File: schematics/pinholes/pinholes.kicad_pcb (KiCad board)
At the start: 2 copper layers, 42 x 10 mm, 3 parts

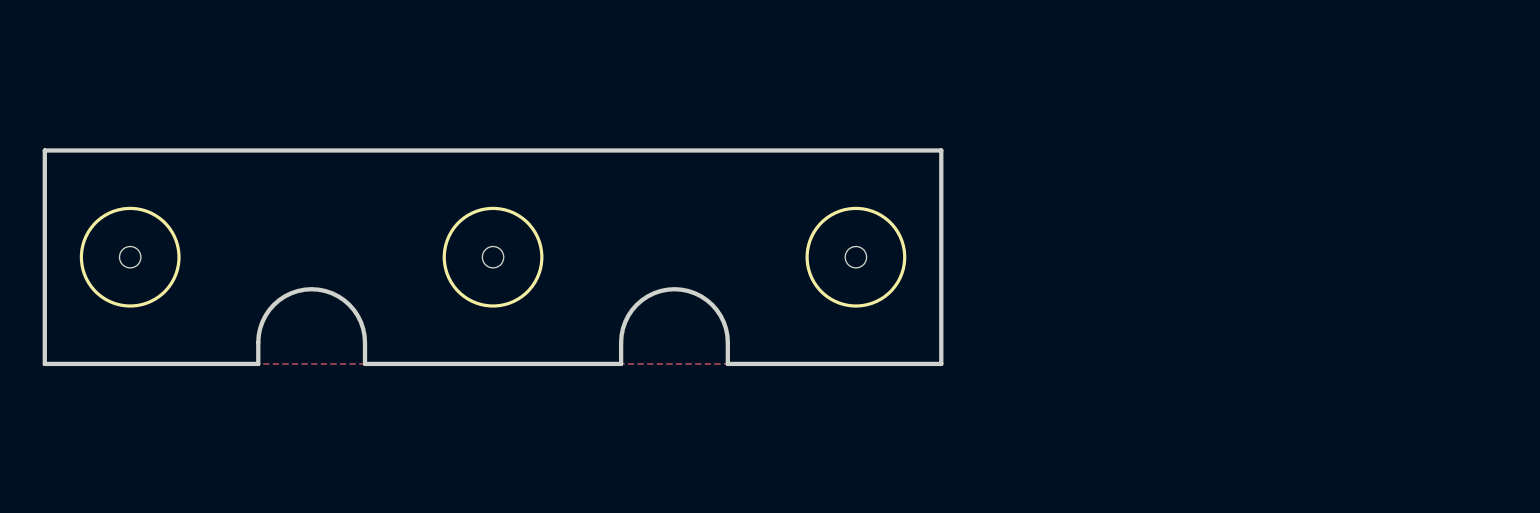
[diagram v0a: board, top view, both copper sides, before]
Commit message: Electronics update for V1
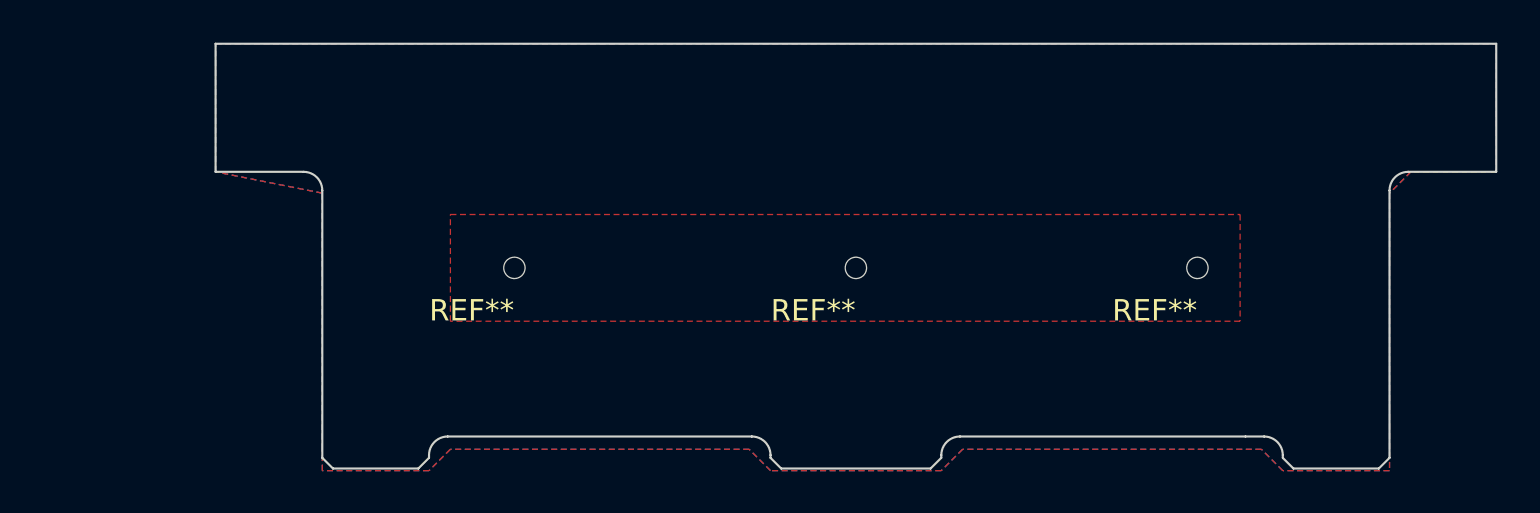
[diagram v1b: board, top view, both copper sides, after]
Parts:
- removed the REF** at (114.0, 105.0)
- removed the REF** at (131.0, 105.0)
- removed the REF** at (148.0, 105.0)
- added REF**: hole, hole, F.Cu at (132.0, 105.5)
- added REF**: hole, hole, F.Cu at (164.0, 105.5)
- added REF**: hole, hole, F.Cu at (148.0, 105.5)
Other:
- board size 42 x 10 mm -> 60 x 19.9 mm
- net class Default: clearance 0 -> 0.2
- rule trace_clearance: 0 -> 0.2
